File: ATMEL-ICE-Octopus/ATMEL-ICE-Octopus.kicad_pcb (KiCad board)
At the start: 2 copper layers, 70.5 x 40 mm, 75 parts, among them J1 ATMEL-ICE SAM SOCKET, J11 ARM Multi-ICE 20-pin JTAG, J12 SWD/JTAG SAM (ARM/Cortex-M db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, J13 SWD/JTAG AVR, J14 aWire/(U)PDI/TPI/debugWire/SP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, J15 SWD, J16 Conn_01x01_Female, J2 ATMEL-ICE AVR SOCKET, J21 Conn_01x03, J22 Conn_01x03, J23 Conn_01x03, J24 Conn_01x03, J3 Angled Conn 1, J4 Angled Conn 2, J5 Angled Conn 3, J8 Conn_01x01_Female, J9 Conn_01x03, Q13 BC846, Q14 BC846, Q15 BC846, Q17 BC846, Q19 Q_PMOS_FDV304P, Q23 BC846, Q24 BC846, Q25 BC846, Q27 BC846, Q29 Q_PMOS_FDV304P, U11 SGM708, U12 TPS2049D, U21 SGM708, U22 TPS2049D

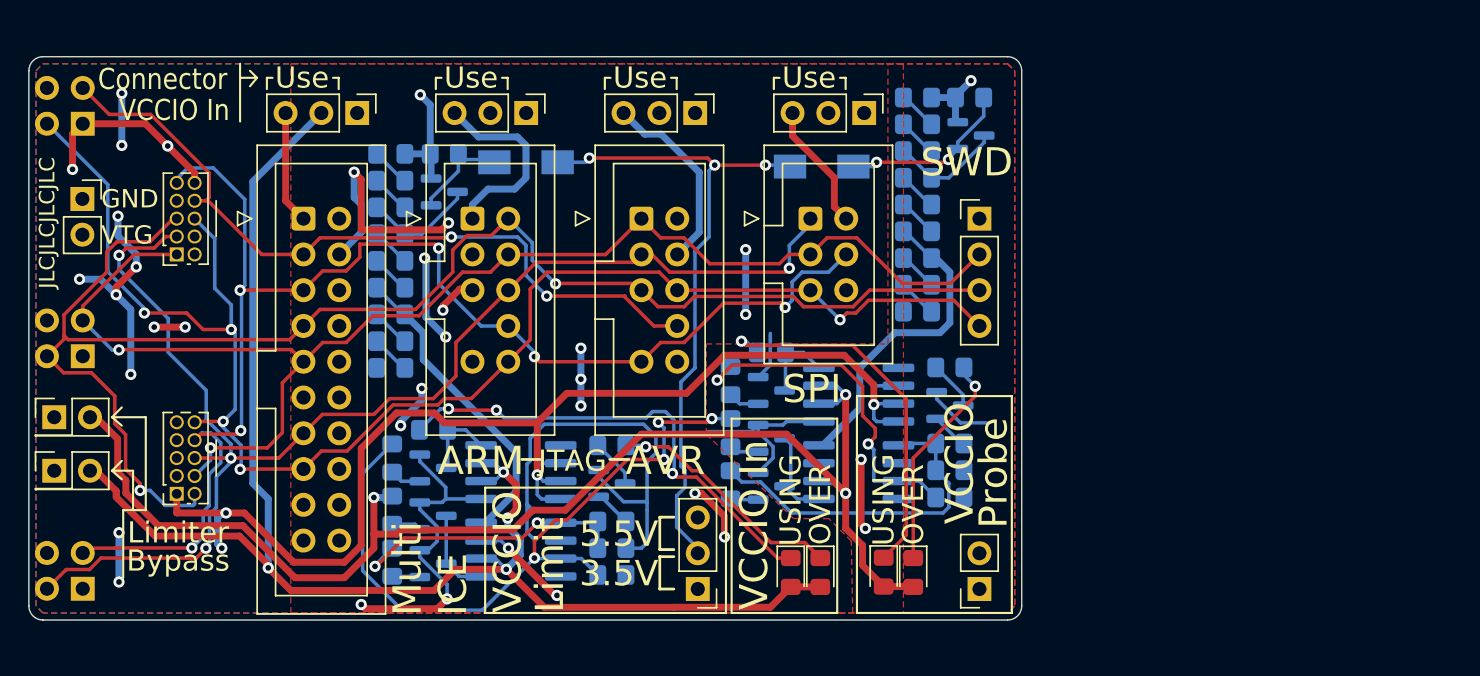
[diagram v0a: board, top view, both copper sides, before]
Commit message: ATMEL-ICE-Octopus: rev B5
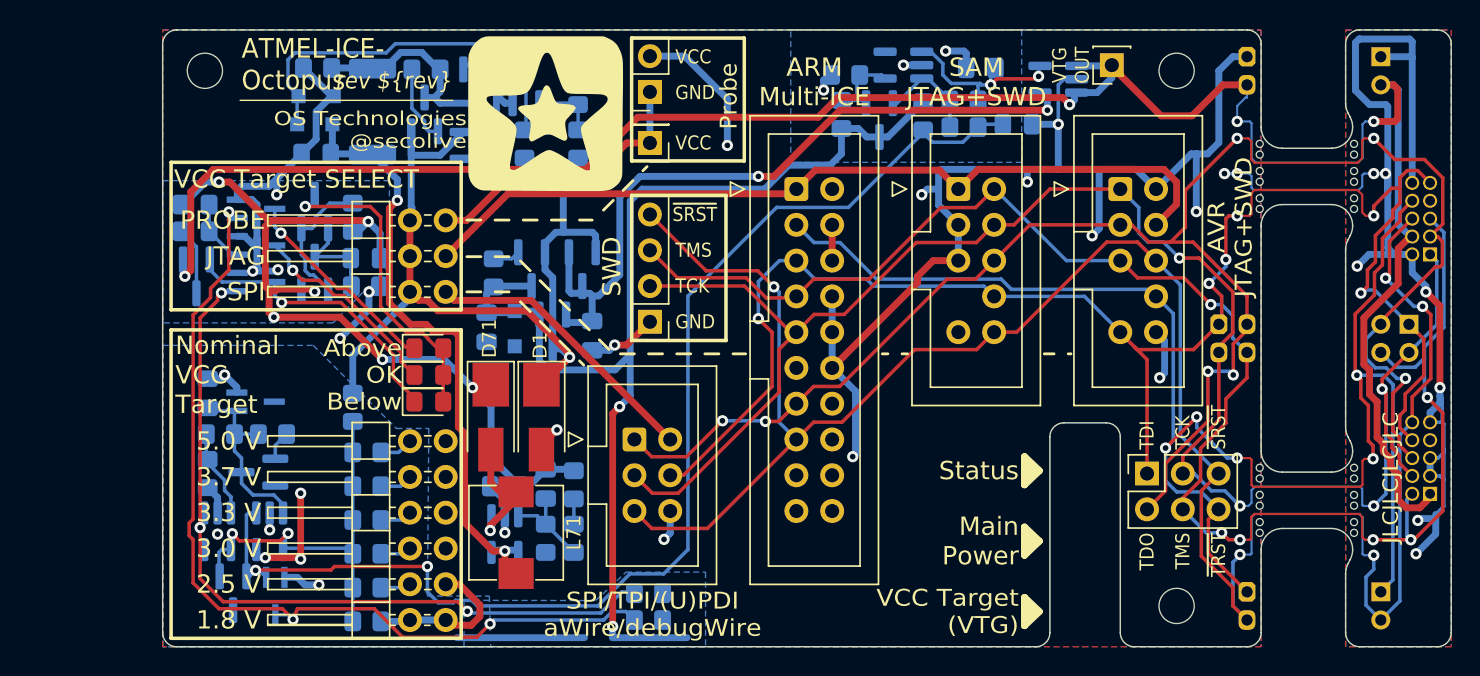
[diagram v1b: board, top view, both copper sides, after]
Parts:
- removed D19, D29: BAT48ZFILM, AA-OSA-Packages:D_MiniMELF
- removed D26: GREEN, LED_SMD:LED_0805_2012Metric_Pad1.15x1.40mm_HandSolder
- removed D28: RED, LED_SMD:LED_0805_2012Metric_Pad1.15x1.40mm_HandSolder
- removed J24: Conn_01x03, Connector_PinHeader_2.54mm:PinHeader_1x03_P2.54mm_Vertical
- removed J3: Angled Conn 1, AA-OSA-connectors:PinHeader_2x02_P2.54mm_Vertical_NoSilk
- removed J4: Angled Conn 2, AA-OSA-connectors:PinHeader_2x02_P2.54mm_Vertical_NoSilk
- removed J5: Angled Conn 3, AA-OSA-connectors:PinHeader_2x02_P2.54mm_Vertical_NoSilk
- removed JP1, JP2: Jumper_2_Open, Connector_PinHeader_2.54mm:PinHeader_2x01_P2.54mm_Vertical
- removed Q13, Q14, Q15, Q17, Q23, Q24, Q25, Q27: BC846, Package_TO_SOT_SMD:SOT-23
- removed Q19, Q29: Q_PMOS_FDV304P, Package_TO_SOT_SMD:SOT-23
- removed R12: 100k, Resistor_SMD:R_0805_2012Metric_Pad1.20x1.40mm_HandSolder
- removed R13, R14, R19, R24, R29: 47k, Resistor_SMD:R_0805_2012Metric_Pad1.20x1.40mm_HandSolder
- removed R15, R17, R25, R27, R44: 22k, Resistor_SMD:R_0805_2012Metric_Pad1.20x1.40mm_HandSolder
- removed R16, R18, R26, R28: 1k, Resistor_SMD:R_0805_2012Metric_Pad1.20x1.40mm_HandSolder
- removed R37, R47: 18k, Resistor_SMD:R_0805_2012Metric_Pad1.20x1.40mm_HandSolder
- removed R38, R48: 1.8k, Resistor_SMD:R_0805_2012Metric_Pad1.20x1.40mm_HandSolder
- removed R43, R46: 28, Resistor_SMD:R_0805_2012Metric_Pad1.20x1.40mm_HandSolder
- removed R45: 470, Resistor_SMD:R_0805_2012Metric_Pad1.20x1.40mm_HandSolder
- removed R49: 220, Resistor_SMD:R_0805_2012Metric_Pad1.20x1.40mm_HandSolder
- removed U11: SGM708, AA-OSA-Packages:SO-8_3.9x4.9mm_P1.27mm
- removed U12, U22: TPS2049D, AA-OSA-Packages:SO-8_3.9x4.9mm_P1.27mm
- added C11: 1u, Capacitor_SMD:C_0805_2012Metric_Pad1.18x1.45mm_HandSolder, B.Cu at (123.0, 99.2)
- added C12: 2.2u, Capacitor_SMD:C_0805_2012Metric_Pad1.18x1.45mm_HandSolder, B.Cu at (130.5, 99.8)
- added C21: 2.2n, Capacitor_SMD:C_0805_2012Metric_Pad1.18x1.45mm_HandSolder, B.Cu at (103.2, 103.9)
- added C51: 33n, Capacitor_SMD:C_0805_2012Metric_Pad1.18x1.45mm_HandSolder, B.Cu at (160.7, 84.8)
- added C53: 1n, Capacitor_SMD:C_0805_2012Metric_Pad1.18x1.45mm_HandSolder, B.Cu at (158.1, 80.8)
- added C66: 1u, Capacitor_SMD:C_0805_2012Metric_Pad1.18x1.45mm_HandSolder, B.Cu at (110.9, 86.9)
- added C71: 1u, Capacitor_SMD:C_0805_2012Metric_Pad1.18x1.45mm_HandSolder, B.Cu at (124.3, 110.5)
- added C72: 10p, Capacitor_SMD:C_0805_2012Metric_Pad1.18x1.45mm_HandSolder, B.Cu at (127.2, 110.3)
- added C85: 1n, Capacitor_SMD:C_0805_2012Metric_Pad1.18x1.45mm_HandSolder, B.Cu at (114.4, 94.3)
- added D1: SMAJ13A, AA-OSA-Packages:D_SMA+SMP_Handsoldering, F.Cu at (126.9, 105.6)
- added D41: BAT54C, AA-OSA-Packages:SOT-23_Handsoldering, B.Cu at (105.0, 118.1)
- added D51: BAT54C, AA-OSA-Packages:SOT-23_Handsoldering, B.Cu at (150.9, 84.5)
- added D61: BAT54S, AA-OSA-Packages:SOT-23_Handsoldering, B.Cu at (122.5, 86.3)
- added D62: PZU5.6B2A, Diode_SMD:D_SOD-323_HandSoldering, B.Cu at (127.6, 86.3)
- added D63: PZU5.6B2A, Diode_SMD:D_SOD-323_HandSoldering, B.Cu at (110.9, 82.8)
- added D64: PZU5.6B2A, Diode_SMD:D_SOD-323_HandSoldering, B.Cu at (110.8, 84.8)
- added D71: SS13, AA-OSA-Packages:D_SMA+SMP_Handsoldering, F.Cu at (123.3, 105.6)
- added D81: RED, LED_SMD:LED_0805_2012Metric_Pad1.15x1.40mm_HandSolder, F.Cu at (118.9, 100.7)
- added D82: GREEN, LED_SMD:LED_0805_2012Metric_Pad1.15x1.40mm_HandSolder, F.Cu at (118.9, 102.6)
- added D83: AMBER, LED_SMD:LED_0805_2012Metric_Pad1.15x1.40mm_HandSolder, F.Cu at (118.9, 104.5)
- added D88: BAT54A, AA-OSA-Packages:SOT-23_Handsoldering, B.Cu at (102.4, 95.6)
- added G1: LOGO, LOGO, F.Cu at (127.2, 84.0)
- added G1: OpenHardware Logo, Symbol:OSHW-Logo2_9.8x8mm_SilkScreen, B.Cu at (156.2, 109.2)
- added G3: KiCad logo, Symbol:KiCad-Logo2_5mm_SilkScreen, B.Cu at (151.9, 97.7)
- added H1: MountingHole, MountingHole:MountingHole_2.5mm, F.Cu at (103.0, 81.0)
- added H2: MountingHole, MountingHole:MountingHole_2.5mm, F.Cu at (172.0, 81.0)
- added H3: MountingHole, MountingHole:MountingHole_2.5mm, F.Cu at (172.0, 119.0)
- added J17: Conn_01x02_Female, Connector_PinSocket_2.54mm:PinSocket_1x02_P2.54mm_Vertical, F.Cu at (134.6, 82.5)
- added J18: conn_02x03_Female, Connector_PinSocket_2.54mm:PinSocket_2x03_P2.54mm_Vertical, F.Cu at (169.9, 109.6)
- added J31: Conn_01x02_Angled, AA-OSA-connectors:PinHeader_1x02_P2.00mm_Angled, B.Cu at (177.0, 80.0)
- added J32: Conn_02x02_Angled, AA-OSA-connectors:PinHeader_2x02_P2.00mm_Angled, B.Cu at (175.0, 99.0)
- added J33: Conn_01x02_Angled, AA-OSA-connectors:PinHeader_1x02_P2.00mm_Angled, B.Cu at (177.0, 118.0)
- added J8: ~, AA-OSA-connectors:PinHeader_2x03_P2.54mm_Horizontal_Jumper, F.Cu at (120.1, 96.7)
- added L71: LQH5BPN100MT0L, AA-OSA-Power:L_6.5x6.5_H4.5, F.Cu at (125.1, 113.8)
- added MB1: Mouse bites, AA-OSA-misc:mouse-bite-3x4mm-slot, F.Cu at (179.5, 88.5)
- added MB2: Mouse bites, AA-OSA-misc:mouse-bite-3x4mm-slot, F.Cu at (183.0, 88.5)
- added MB3: Mouse bites, AA-OSA-misc:mouse-bite-3x4mm-slot, F.Cu at (179.5, 111.5)
- added MB4: Mouse bites, AA-OSA-misc:mouse-bite-3x4mm-slot, F.Cu at (183.0, 111.5)
- added Q11: CPH3910, AA-OSA-Packages:SOT-23_Handsoldering, B.Cu at (126.2, 95.1)
- added Q12: CPH3910, AA-OSA-Packages:SOT-23_Handsoldering, B.Cu at (129.8, 95.1)
- added Q21: 2SK2394, AA-OSA-Packages:SOT-23_Handsoldering, B.Cu at (106.8, 109.5)
- added Q41: NX6008NBKW, Package_TO_SOT_SMD:SOT-323_SC-70_Handsoldering, B.Cu at (108.0, 118.3)
- added Q61: CPH3910, AA-OSA-Packages:SOT-23_Handsoldering, B.Cu at (118.6, 84.1)
- added Q62: NXV100XP, AA-OSA-Packages:SOT-23_Handsoldering, B.Cu at (122.3, 82.1)
- added Q63: BC857B, AA-OSA-Packages:SOT-23_Handsoldering, B.Cu at (125.8, 82.1)
- added Q81: NX6008NBKW, Package_TO_SOT_SMD:SOT-323_SC-70_Handsoldering, B.Cu at (106.6, 90.8)
- added Q82: NX6008NBKW, Package_TO_SOT_SMD:SOT-323_SC-70_Handsoldering, B.Cu at (106.6, 93.4)
- added Q83: NX6008NBKW, Package_TO_SOT_SMD:SOT-323_SC-70_Handsoldering, B.Cu at (106.6, 96.0)
- added Q84: BC857B, AA-OSA-Packages:SOT-23_Handsoldering, B.Cu at (110.8, 91.0)
- added Q85: BC857B, AA-OSA-Packages:SOT-23_Handsoldering, B.Cu at (110.8, 95.4)
- added R51: 180k, Resistor_SMD:R_0805_2012Metric_Pad1.20x1.40mm_HandSolder, B.Cu at (154.0, 84.2)
- added R52: 33k, Resistor_SMD:R_0805_2012Metric_Pad1.20x1.40mm_HandSolder, B.Cu at (156.9, 85.0)
- added R53: 390k, Resistor_SMD:R_0805_2012Metric_Pad1.20x1.40mm_HandSolder, B.Cu at (156.9, 83.1)
- added R54: 180k, Resistor_SMD:R_0805_2012Metric_Pad1.20x1.40mm_HandSolder, B.Cu at (148.5, 81.3)
- added R55: 120k, Resistor_SMD:R_0805_2012Metric_Pad1.20x1.40mm_HandSolder, B.Cu at (148.2, 84.1)
- added R61: 150, Resistor_SMD:R_0805_2012Metric_Pad1.20x1.40mm_HandSolder, B.Cu at (118.7, 80.9)
- added R62: 82k, Resistor_SMD:R_0805_2012Metric_Pad1.20x1.40mm_HandSolder, B.Cu at (125.7, 86.2)
- added R63: 82k, Resistor_SMD:R_0805_2012Metric_Pad1.20x1.40mm_HandSolder, B.Cu at (129.5, 82.4)
- added R64: 82k, Resistor_SMD:R_0805_2012Metric_Pad1.20x1.40mm_HandSolder, B.Cu at (129.5, 86.2)
- added R65: 680k, Resistor_SMD:R_0805_2012Metric_Pad1.20x1.40mm_HandSolder, B.Cu at (111.0, 80.8)
- added R66: 10 2W, Resistor_SMD:R_2512_6332Metric_Pad1.40x3.35mm_HandSolder, B.Cu at (114.9, 83.9)
- added R71: 220k, Resistor_SMD:R_0805_2012Metric_Pad1.20x1.40mm_HandSolder, B.Cu at (127.2, 114.2)
- added R72: 330k, Resistor_SMD:R_0805_2012Metric_Pad1.20x1.40mm_HandSolder, B.Cu at (129.2, 114.2)
- added R73: 39k, Resistor_SMD:R_0805_2012Metric_Pad1.20x1.40mm_HandSolder, B.Cu at (129.2, 110.4)
- added R84: 47k, Resistor_SMD:R_0805_2012Metric_Pad1.20x1.40mm_HandSolder, B.Cu at (114.4, 96.3)
- added R85: 280, Resistor_SMD:R_0805_2012Metric_Pad1.20x1.40mm_HandSolder, B.Cu at (113.5, 91.4)
- added R88: 6.8k, Resistor_SMD:R_0805_2012Metric_Pad1.20x1.40mm_HandSolder, B.Cu at (102.3, 92.4)
- added R89: 680k, Resistor_SMD:R_0805_2012Metric_Pad1.20x1.40mm_HandSolder, B.Cu at (102.3, 90.5)
- added U41: NCS2202SN2T1, AA-OSA-Packages:SOT-23-5_HandSoldering, B.Cu at (107.6, 113.7)
- added U42: NCS2202SN2T1, AA-OSA-Packages:SOT-23-5_HandSoldering, B.Cu at (103.9, 113.7)
- added U51: NCS2200SN2T1, AA-OSA-Packages:SOT-23-5_HandSoldering, B.Cu at (152.6, 80.6)
- added U52: AP2280-xW, AA-OSA-Packages:SOT-23-5_HandSoldering, B.Cu at (163.6, 81.6)
- added U71: AP3015A, AA-OSA-Packages:SOT-23-5_HandSoldering, B.Cu at (124.3, 113.9)
- D11: value GREEN -> PZU5.6B2A; footprint LED_SMD:LED_0805_2012Metric_Pad1.15x1.40mm_HandSolder -> Diode_SMD:D_SOD-323_HandSoldering; moved to B.Cu
- D12: value RED -> BAT54C; footprint LED_SMD:LED_0805_2012Metric_Pad1.15x1.40mm_HandSolder -> AA-OSA-Packages:SOT-23_Handsoldering; moved to B.Cu
- J1: value ATMEL-ICE SAM SOCKET -> conn_02x05; moved to B.Cu
- J11: value ARM Multi-ICE 20-pin JTAG -> conn_02x10
- J12: value SWD/JTAG SAM (ARM/Cortex-M dbg) -> conn_02x05_key7
- J13: value SWD/JTAG AVR -> conn_02x05_key7
- J14: value aWire/(U)PDI/TPI/debugWire/SPI Target -> conn_02x03
- J15: value SWD -> conn_01x04
- J16: value Conn_01x01_Female -> conn_01x01; footprint Connector_PinSocket_2.54mm:PinSocket_1x02_P2.54mm_Vertical -> Connector_PinHeader_2.54mm:PinHeader_1x01_P2.54mm_Vertical
- J2: value ATMEL-ICE AVR SOCKET -> conn_02x05; moved to B.Cu
- J21, J23: value Conn_01x03 -> Conn_01x02_Angled; footprint Connector_PinHeader_2.54mm:PinHeader_1x03_P2.54mm_Vertical -> Connector_PinHeader_2.00mm:PinHeader_1x02_P2.00mm_Horizontal; moved to B.Cu
- J22: value Conn_01x03 -> Conn_02x02_Angled; footprint Connector_PinHeader_2.54mm:PinHeader_1x03_P2.54mm_Vertical -> Connector_PinHeader_2.00mm:PinHeader_2x02_P2.00mm_Horizontal; moved to B.Cu
- J6: renamed from J8; footprint Connector_PinSocket_2.54mm:PinSocket_1x02_P2.54mm_Vertical -> Connector_PinSocket_2.54mm:PinSocket_1x01_P2.54mm_Vertical
- J9: value Conn_01x03 -> ~; footprint Connector_PinHeader_2.54mm:PinHeader_1x03_P2.54mm_Vertical -> AA-OSA-connectors:PinHeader_2x06_P2.54mm_Horizontal_Jumper
- R11: value 100k -> 560
- R21: value 100k -> 6.8k
- R22: value 100k -> 13k0 0.1%
- R23: value 47k -> 72k3 0.1%
- R31: value 12k -> 85k6 0.1%
- R32: value 470 -> 80k6 0.1%
- R33: value 28 -> 48k7 0.1%
- R34: value 22k -> 37k4 0.1%
- R35: value 470 -> 30k1 0.1%
- R36: value 28 -> 17k4 0.1%
- R39: value 220 -> 48k1 0.1%
- R41: value 12k -> 47k
- R42: value 470 -> 47k
- U21: value SGM708 -> TS4061BICT; footprint AA-OSA-Packages:SO-8_3.9x4.9mm_P1.27mm -> Package_TO_SOT_SMD:SOT-323_SC-70_Handsoldering
- moved J1 89.0 mm to (190.0, 111.0), turned to 0 degrees
- moved J2 89.0 mm to (190.0, 94.0), turned to 0 degrees
- moved J6 73.7 mm to (167.4, 80.6), turned to 180 degrees
- moved J21 72.8 mm to (186.5, 80.0), turned to 180 degrees
- moved J22 64.5 mm to (188.5, 99.0), turned to 180 degrees
- moved J23 59.4 mm to (186.5, 118.0), turned to 180 degrees
- moved R39 45.7 mm to (113.5, 104.9), turned to 90 degrees
- moved R31 44.9 mm to (114.5, 120.1), turned to 180 degrees
- moved R32 44.6 mm to (114.5, 117.7), turned to 180 degrees
- moved R33 44.4 mm to (114.5, 115.3), turned to 180 degrees
- moved R34 44.1 mm to (114.5, 112.9), turned to 180 degrees
- moved R35 43.9 mm to (114.5, 110.5), turned to 180 degrees
- moved R36 43.7 mm to (114.5, 108.1), turned to 180 degrees
- moved J16 39.4 mm to (134.6, 86.1)
- moved R11 36.1 mm to (123.5, 95.3), turned to 90 degrees
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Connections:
- D11 pad 1: Net-(D11-Pad1) -> VAA
- D11 pad 2: VDD_RED -> GND
- D12 pad 1: Net-(D12-Pad1) -> VAA
- D12 pad 2: VDD_RED -> /VoltageLimiter/VIN_SLOW
- J11 pad 1: /VIN1 -> /VIN_JTAG
- J12 pad 1: /VIN2 -> /VIN_JTAG
- J13 pad 4: /VIN3 -> /VIN_JTAG
- J14 pad 2: /VIN4 -> /VIN_AVR
- J16 pad 1: VDD_RED -> /VIN_PROBE
- J21 pad 1: unconnected-(J21-Pad1) -> GND
- J21 pad 2: VDD_BLACK -> /VTG
- J22 pad 1: unconnected-(J22-Pad1) -> /TDI
- J22 pad 2: VDD_BLACK -> /TDO
- J22 pad 3: /VIN2 -> /TCK
- J23 pad 1: unconnected-(J23-Pad1) -> /nTRST
- J23 pad 2: VDD_BLACK -> /nSRST
- J6 pad 1: GND -> /VTG
- J9 pad 2: /~{LIMIT_LOW} -> GND
- J9 pad 3: unconnected-(J9-Pad3) -> GND
- R11 pad 1: /USE_RED -> VAA
- R11 pad 2: GND -> Net-(Q11-Pad1)
- R21 pad 1: /USE_BLACK -> /VoltageLimiter/VREF_1v25
- R21 pad 2: GND -> Net-(Q21-Pad1)
- R22 pad 1: /BLACK_OVERVOLTAGE -> /VoltageLimiter/VREF_1v25
- R22 pad 2: GND -> /VoltageLimiter/VREF_1v06
- R23 pad 1: /BLACK_OVERVOLTAGE -> /VoltageLimiter/VREF_1v06
- R23 pad 2: Net-(Q23-Pad1) -> GND
- R31 pad 2: Net-(R31-Pad2) -> /VoltageLimiter/VIN_SCALED
- R32 pad 1: Net-(R31-Pad2) -> /VoltageLimiter/D_2V5
- R32 pad 2: Net-(R32-Pad2) -> /VoltageLimiter/VIN_SCALED
- R33 pad 1: Net-(R32-Pad2) -> /VoltageLimiter/D_3V0
- R33 pad 2: /RED_SENSE -> /VoltageLimiter/VIN_SCALED
- R34 pad 1: /RED_SENSE -> /VoltageLimiter/D_3V3
- R34 pad 2: Net-(R34-Pad2) -> /VoltageLimiter/VIN_SCALED
- R35 pad 1: Net-(R34-Pad2) -> /VoltageLimiter/D_3V7
- R35 pad 2: Net-(R35-Pad2) -> /VoltageLimiter/VIN_SCALED
- R36 pad 1: Net-(R35-Pad2) -> /VoltageLimiter/D_5V0
- R36 pad 2: Net-(Q19-Pad3) -> /VoltageLimiter/VIN_SCALED
- R39 pad 1: Net-(R38-Pad2) -> /VoltageLimiter/VIN_SCALED
- R39 pad 2: VDD_RED -> /VIN
- R41 pad 1: GND -> VAA
- R41 pad 2: Net-(R41-Pad2) -> /VIN_ABOVE
- R42 pad 1: Net-(R41-Pad2) -> VAA
- R42 pad 2: Net-(R42-Pad2) -> /VIN_BELOW
- U21 pad 1: Net-(Q23-Pad3) -> /VoltageLimiter/VREF_1v25
- U21 pad 2: VDD_BLACK -> GND
- U21 pad 3: GND -> unconnected-(U21-Pad3)
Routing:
- net VDD_BLACK: track 130.8 -> 0.00 mm, vias 14 -> 0
- net GND: track 128.1 -> 250.3 mm, vias 15 -> 33
- net VDD_RED: track 98.7 -> 0.00 mm, vias 4 -> 0
- net VAA: track 0.00 -> 97.2 mm, vias 0 -> 5
- net /VoltageLimiter/aENABLE: track 0.00 -> 87.6 mm, vias 0 -> 2
- net /VIN: track 0.00 -> 70.9 mm, vias 0 -> 1
- net /VIN_ABOVE: track 0.00 -> 63.8 mm, vias 0 -> 3
- net /VLED: track 0.00 -> 60.3 mm, vias 0 -> 6
- net /VIN_JTAG: track 0.00 -> 59.1 mm
- net /nTRST: track 53.8 -> 112.1 mm, vias 2 -> 5
- net /VIN_BELOW: track 0.00 -> 54.5 mm, vias 0 -> 3
- net /VoltageLimiter/VIN_SLOW: track 0.00 -> 51.0 mm, vias 0 -> 2
- net /USE_BLACK: track 50.6 -> 0.00 mm, vias 4 -> 0
- net /nSRST: track 108.1 -> 156.1 mm
- net /~{LIMIT_LOW}: track 46.1 -> 0.00 mm, vias 3 -> 0
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- added copper zone on B.Cu, net /VLED
- added copper zone on F.Cu, net GND
- added copper zone on B.Cu, net VAA
- removed copper zone on F.Cu, net /VTG
- removed copper zone on F.Cu, net VDD_BLACK
- removed copper zone on F.Cu, net VDD_RED
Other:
- board size 70.5 x 40 mm -> 91.5 x 43.8 mm
- board text added: "1.8 V"
- board text added: "2.5 V"
- board text added: "3.0 V"
- board text added: "3.3 V"
- board text added: "3.7 V"
- board text added: "5.0 V"
- board text added: "ARM Multi-ICE"
- board text added: "ATMEL-ICE- Octopus"
- board text added: "AVR JTAG+SWD"
- board text added: "Above"
- board text added: "Atmel-ICE PCB"
- board text added: "Atmel-ICE PCB Edge"
- board text added: "Below"
- board text added: "Connecting PCB"
- board text added: "Licensed under CERN-OHL-W v2 https://ohwr.org/cernohl"
- board text added: "Main Power"
- board text added: "Nominal VCC Target"
- board text added: "OK"
- board text added: "OS Technologies @secolive"
- board text added: "Octopus PCB"
- board text added: "PROBE"
- board text added: "SAM JTAG+SWD"
- board text added: "SPI/TPI/(U)PDI aWire/debugWire"
- board text added: "Source: https://github.com/secolive/"
- board text added: "Status"
- board text added: "TCK"
- board text added: "TDI"
- board text added: "TDO"
- board text added: "TMS"
- board text added: "VCC"
- board text added: "VCC Target (VTG)"
- board text added: "VCC Target SELECT"
- board text added: "VTG OUT"
- board text added: "~{SRST}"
- board text added: "~{TRST}"
- board text removed: "${license}"
- board text removed: "3.5V"
- board text removed: "5.5V"
- board text removed: "ARM"
- board text removed: "ATMEL-ICE-Octopus"
- board text removed: "AVR"
- board text removed: "Bypass"
- board text removed: "Connector"
- board text removed: "Limit"
- board text removed: "Limiter"
- board text removed: "Multi ICE"
- board text removed: "OVER"
- board text removed: "USING"
- board text removed: "Use"
- board text removed: "VCCIO"
- board text removed: "VCCIO In"
- board text removed: "VTG"
